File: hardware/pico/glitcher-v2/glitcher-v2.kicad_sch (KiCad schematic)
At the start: 6 parts, among them J1 UART Connector, J2 PMBUS Connector, J3 Flash Conn L, J4 Flash Conn R, U1 TXS0102, U2 Pico

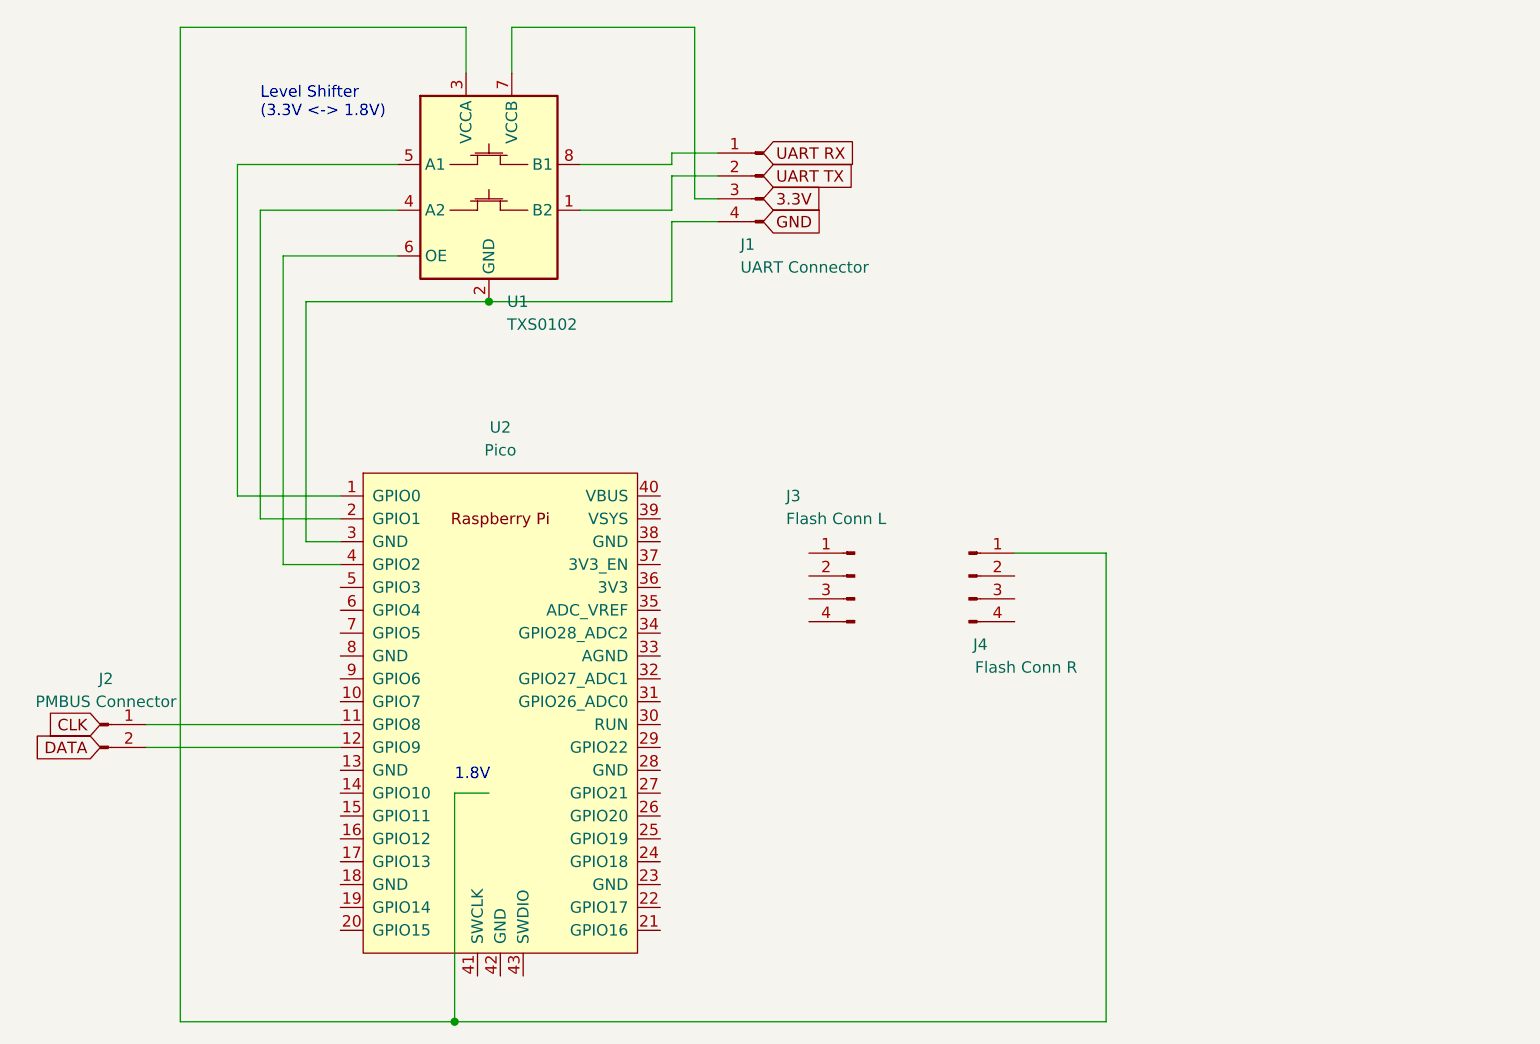
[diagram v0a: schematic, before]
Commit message: Moar pico schematics + docs
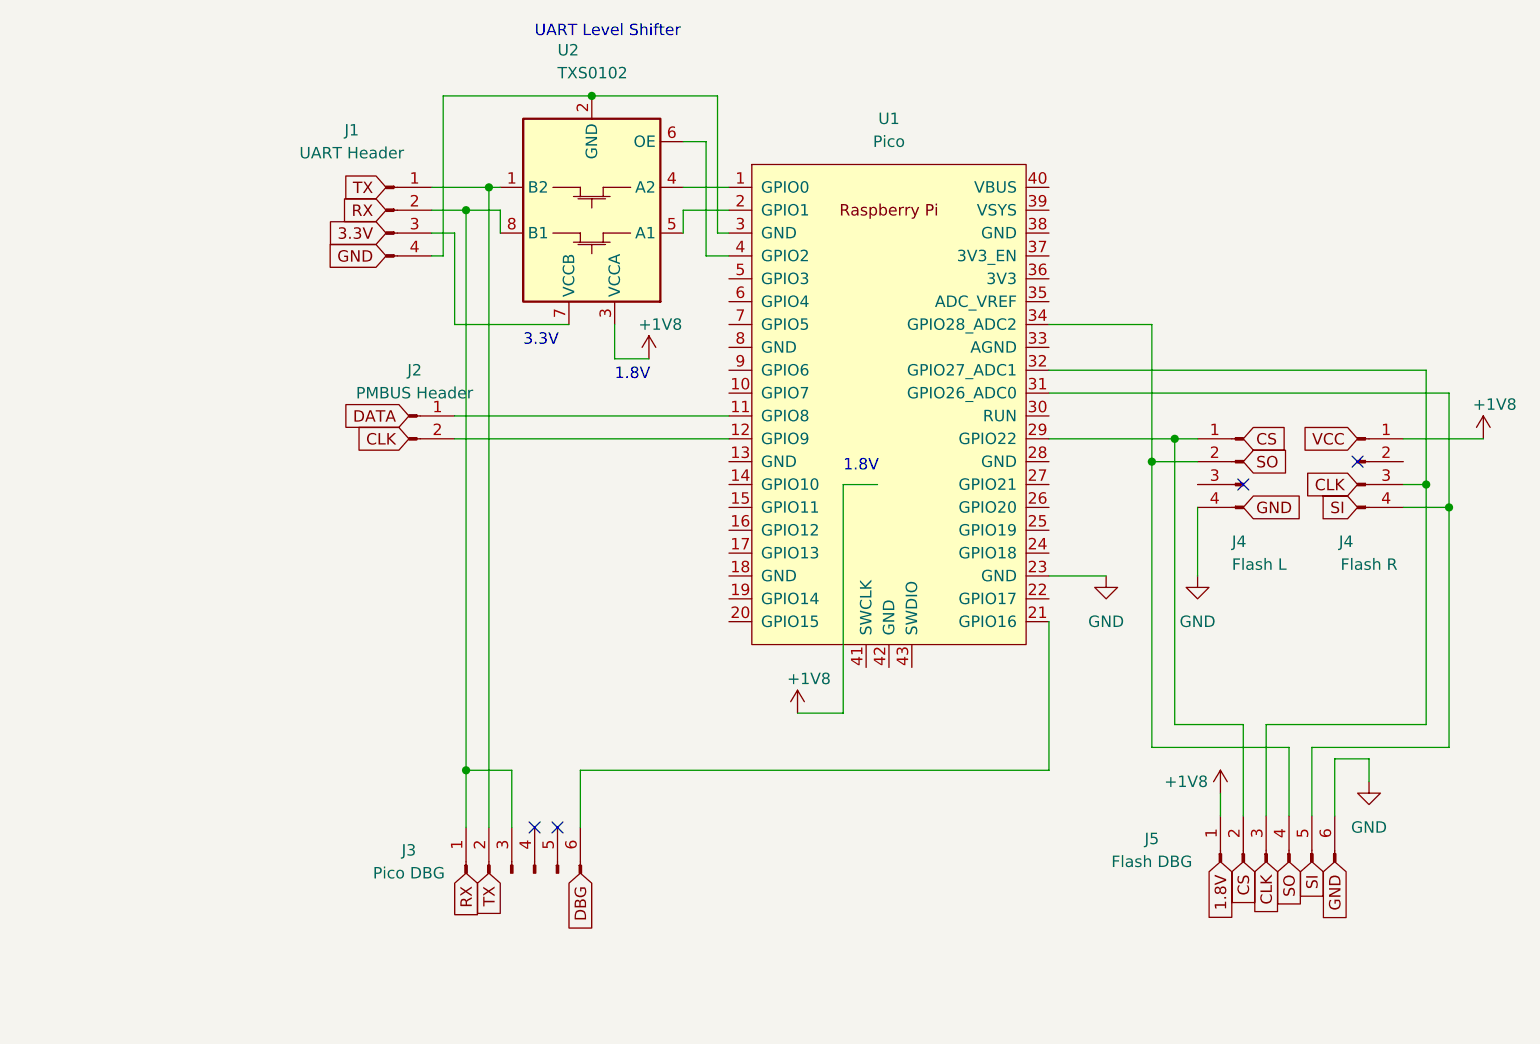
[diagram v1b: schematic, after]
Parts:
- removed U1: TXS0102, Package_SO:VSSOP-8_2.3x2mm_P0.5mm, symbol Logic_LevelTranslator:TXS0102DCU
- added J3: Pico DBG, symbol Connector:Conn_01x06_Male
- added J5: Flash DBG, symbol Connector:Conn_01x06_Male
- added U2: TXS0102, Package_SO:VSSOP-8_2.3x2mm_P0.5mm, symbol Logic_LevelTranslator:TXS0102DCU
- J1: value UART Connector -> UART Header
- J2: value PMBUS Connector -> PMBUS Header
- J4: renamed from J3; value Flash Conn L -> Flash L
- J4: value Flash Conn R -> Flash R
- renumbered U2 to U1
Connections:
- net GND: now also J4.4 (Pin_4), U1.23 (GND), J5.6 (Pin_6)
- net at U1.1 (GPIO0): now also U2.4 (A2)
- net at U1.2 (GPIO1): now also U2.5 (A1)
- net at U1.21 (GPIO16): now also J3.6 (Pin_6)
- net at U1.29 (GPIO22): now also J4.1 (Pin_1), J5.2 (Pin_2)
- net at J1.4 (Pin_4), U1.3 (GND): now also U2.2 (GND)
- net at U1.31 (GPIO26_ADC0): now also J4.4 (Pin_4), J5.5 (Pin_5)
- net at U1.32 (GPIO27_ADC1): now also J4.3 (Pin_3), J5.3 (Pin_3)
- net at U1.34 (GPIO28_ADC2): now also J4.2 (Pin_2), J5.4 (Pin_4)
- net at U1.4 (GPIO2): now also U2.6 (OE)
- net at J1.2 (Pin_2): now also J3.1 (Pin_1), J3.3 (Pin_3), U2.8 (B1)
- net +1V8: now reaches J4.1 (Pin_1)
- net +1V8: now also J5.1 (Pin_1), U2.3 (VCCA)
- net at J1.3 (Pin_3): now also U2.7 (VCCB)
- net at J1.1 (Pin_1): now also J3.2 (Pin_2), U2.1 (B2)
- no-connect marks 0 -> 4
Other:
- note added: "3.3V"
- note added: "UART Level Shifter"
- note removed: "Level Shifter (3.3V <-> 1.8V)"
- moved on the sheet: J2, J4, U1
